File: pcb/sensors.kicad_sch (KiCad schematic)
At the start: 7 parts, among them U3 BME280, U4 SGP40

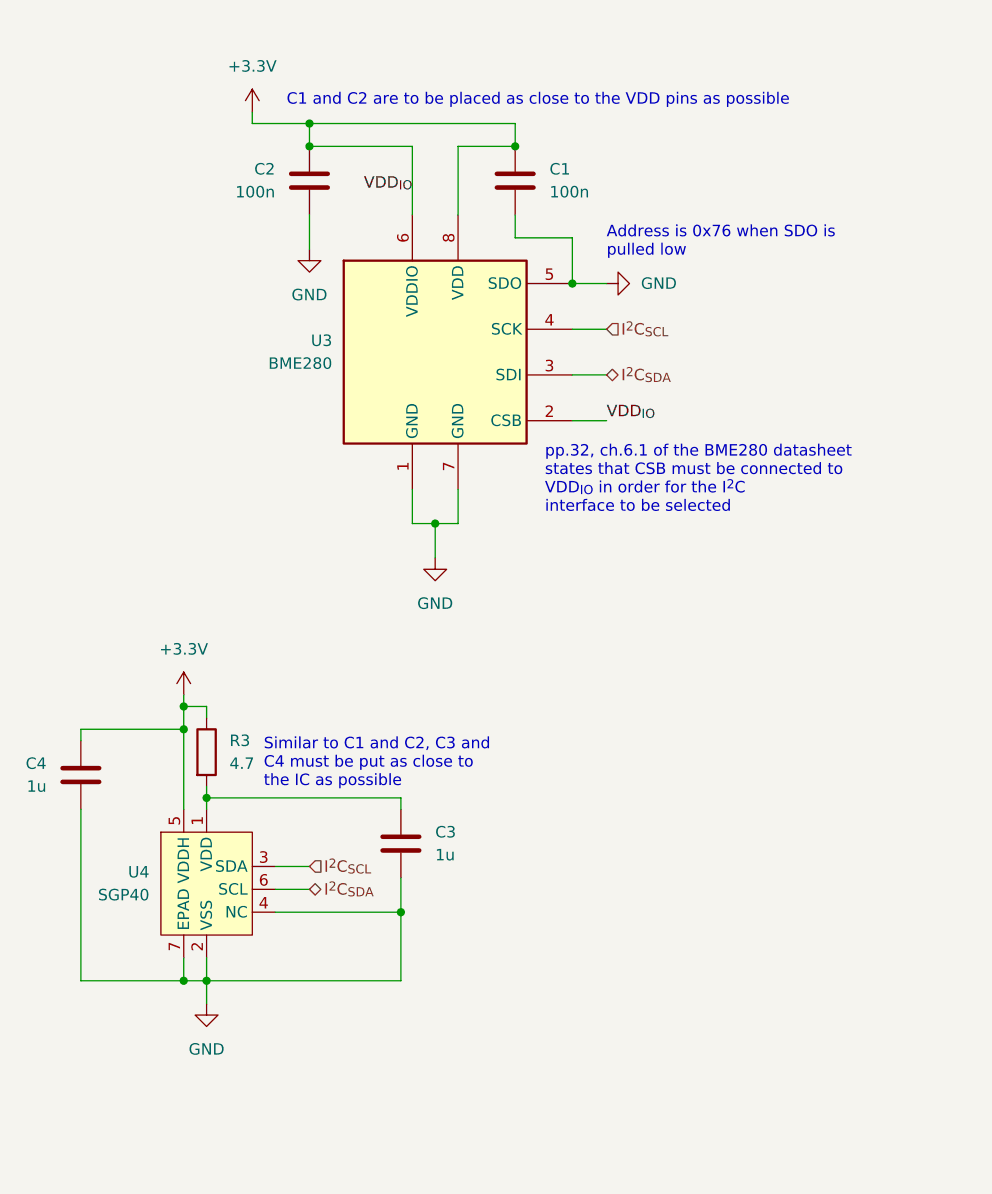
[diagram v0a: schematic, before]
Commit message: chore: organization
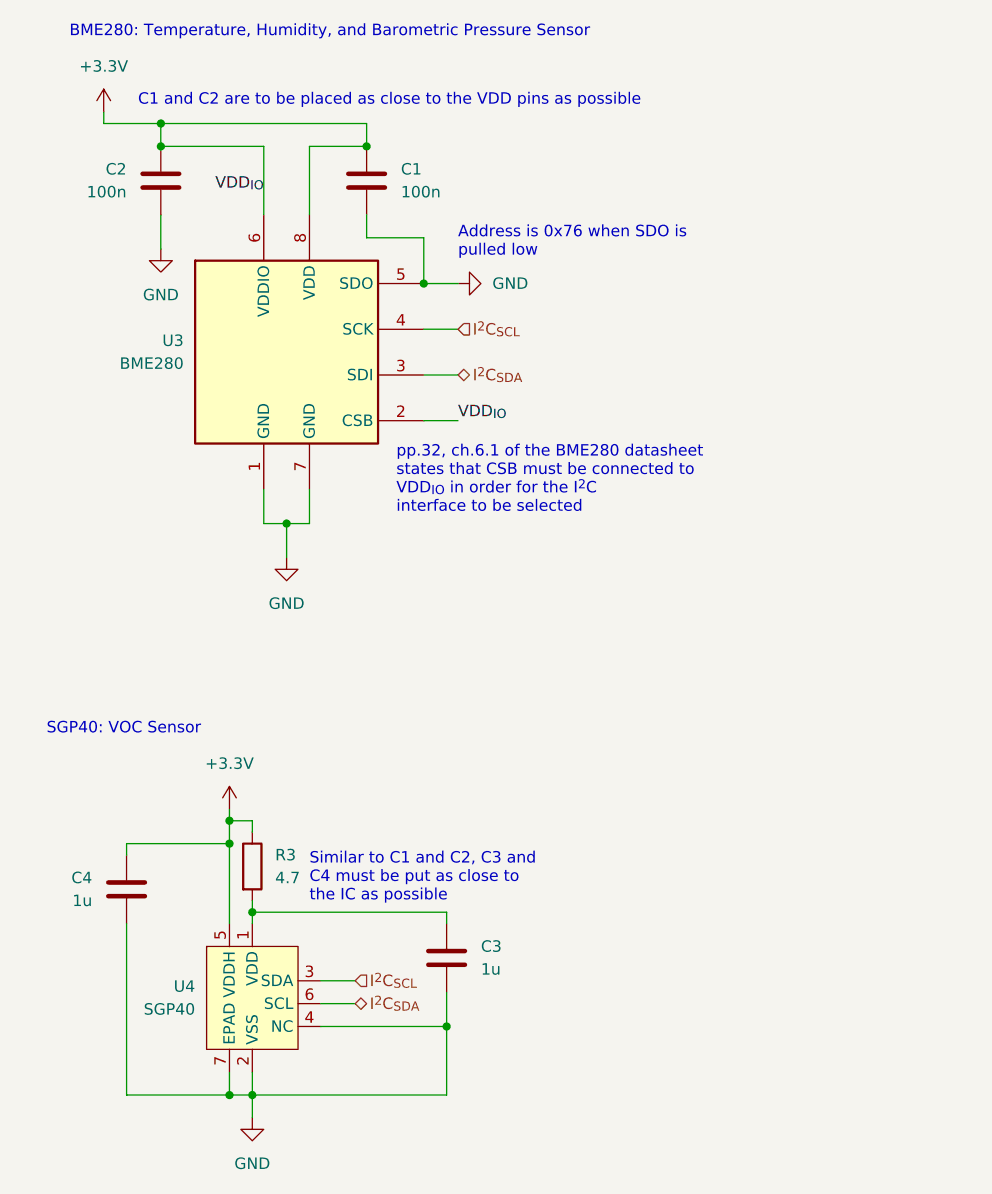
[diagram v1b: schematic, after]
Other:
- note added: "BME280: Temperature, Humidity, and Barometric Pressure Sensor"
- note added: "SGP40: VOC Sensor"
- moved on the sheet: C1, C2, C3, C4, R3, U3, U4
